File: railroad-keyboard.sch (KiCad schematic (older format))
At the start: 208 parts, among them SW1 SW_Push, U1 ATmega32U4-AU, Y1 16MHz

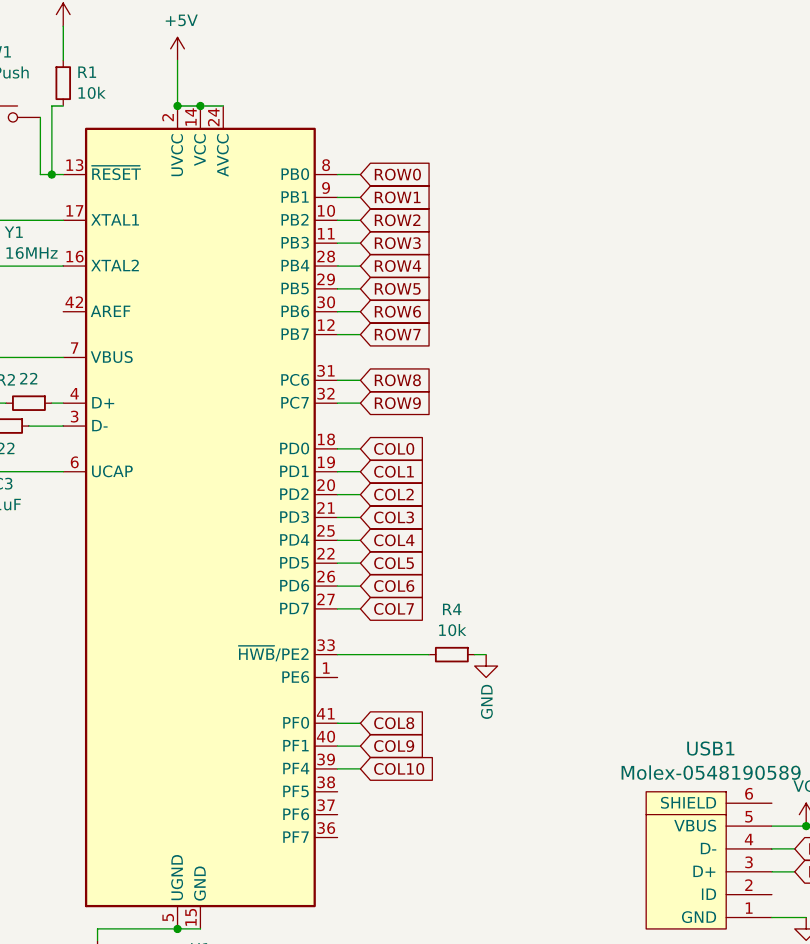
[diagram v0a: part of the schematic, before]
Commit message: Completion of first draft
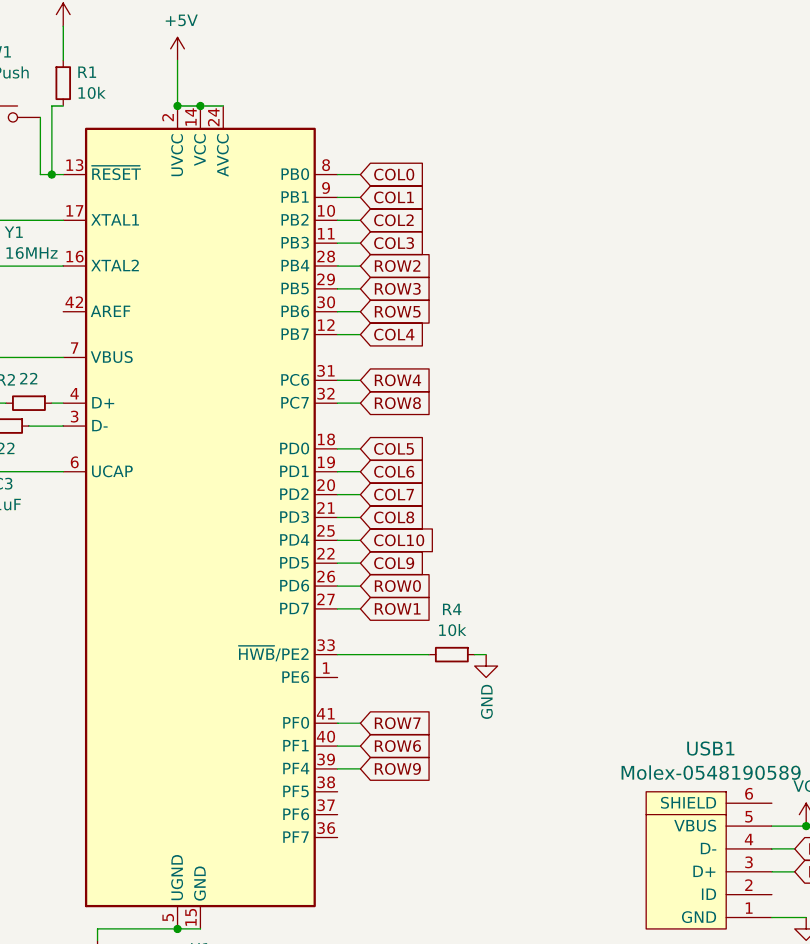
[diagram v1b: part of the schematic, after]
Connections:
- net COL0: now also U1.8 (PB0); no longer U1.18 (PD0)
- net COL1: now also U1.9 (PB1); no longer U1.19 (PD1)
- net COL10: now also U1.25 (PD4); no longer U1.39 (PF4)
- net COL2: now also U1.10 (PB2); no longer U1.20 (PD2)
- net COL3: now also U1.11 (PB3); no longer U1.21 (PD3)
- net COL4: now also U1.12 (PB7); no longer U1.25 (PD4)
- net COL5: now also U1.18 (PD0); no longer U1.22 (PD5)
- net COL6: now also U1.19 (PD1); no longer U1.26 (PD6)
- net COL7: now also U1.20 (PD2); no longer U1.27 (PD7)
- net COL8: now also U1.21 (PD3); no longer U1.41 (PF0)
- net COL9: now also U1.22 (PD5); no longer U1.40 (PF1)
- net ROW0: now also U1.26 (PD6); no longer U1.8 (PB0)
- net ROW1: now also U1.27 (PD7); no longer U1.9 (PB1)
- net ROW2: now also U1.28 (PB4); no longer U1.10 (PB2)
- net ROW3: now also U1.29 (PB5); no longer U1.11 (PB3)
- net ROW4: now also U1.31 (PC6); no longer U1.28 (PB4)
- net ROW5: now also U1.30 (PB6); no longer U1.29 (PB5)
- net ROW6: now also U1.40 (PF1); no longer U1.30 (PB6)
- net ROW7: now also U1.41 (PF0); no longer U1.12 (PB7)
- net ROW8: now also U1.32 (PC7); no longer U1.31 (PC6)
- net ROW9: now also U1.39 (PF4); no longer U1.32 (PC7)
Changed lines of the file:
@@
 Wire Wire Line
 	17000 4350 17000 7350
-Text GLabel 2850 12200 2    50   Input ~ 0
+Text GLabel 2850 14000 2    50   Input ~ 0
 ROW1
-Text GLabel 2850 12100 2    50   Input ~ 0
+Text GLabel 2850 13900 2    50   Input ~ 0
 ROW0
-Text GLabel 2850 12400 2    50   Input ~ 0
+Text GLabel 2850 12600 2    50   Input ~ 0
 ROW3
-Text GLabel 2850 12300 2    50   Input ~ 0
+Text GLabel 2850 12500 2    50   Input ~ 0
 ROW2
-Text GLabel 2850 12600 2    50   Input ~ 0
+Text GLabel 2850 12700 2    50   Input ~ 0
 ROW5
-Text GLabel 2850 12500 2    50   Input ~ 0
+Text GLabel 2850 13000 2    50   Input ~ 0
 ROW4
-Text GLabel 2850 12800 2    50   Input ~ 0
+Text GLabel 2850 14500 2    50   Input ~ 0
 ROW7
-Text GLabel 2850 12700 2    50   Input ~ 0
+Text GLabel 2850 14600 2    50   Input ~ 0
 ROW6
+Text GLabel 2850 14700 2    50   Input ~ 0
+ROW9
 Text GLabel 2850 13100 2    50   Input ~ 0
-ROW9
-Text GLabel 2850 13000 2    50   Input ~ 0
 ROW8
 Wire Wire Line
@@
 Wire Wire Line
 	2850 12200 2750 12200
+Text GLabel 2850 12100 2    50   Input ~ 0
+COL0
+Text GLabel 2850 12200 2    50   Input ~ 0
+COL1
+Text GLabel 2850 12300 2    50   Input ~ 0
+COL2
+Text GLabel 2850 12400 2    50   Input ~ 0
+COL3
+Text GLabel 2850 12800 2    50   Input ~ 0
+COL4
 Text GLabel 2850 13300 2    50   Input ~ 0
-COL0
+COL5
+Text GLabel 2850 13500 2    50   Input ~ 0
+COL7
+Text GLabel 2850 13600 2    50   Input ~ 0
+COL8
+Text GLabel 2850 13800 2    50   Input ~ 0
+COL9
+Text GLabel 2850 13700 2    50   Input ~ 0
+COL10
 Text GLabel 2850 13400 2    50   Input ~ 0
-COL1
-Text GLabel 2850 13500 2    50   Input ~ 0
-COL2
-Text GLabel 2850 13600 2    50   Input ~ 0
-COL3
-Text GLabel 2850 13700 2    50   Input ~ 0
-COL4
-Text GLabel 2850 13800 2    50   Input ~ 0
-COL5
-Text GLabel 2850 14000 2    50   Input ~ 0
-COL7
-Text GLabel 2850 14500 2    50   Input ~ 0
-COL8
-Text GLabel 2850 14600 2    50   Input ~ 0
-COL9
-Text GLabel 2850 14700 2    50   Input ~ 0
-COL10
-Text GLabel 2850 13900 2    50   Input ~ 0
 COL6
 Wire Wire Line
